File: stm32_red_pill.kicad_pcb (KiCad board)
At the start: 4 copper layers, 59 x 31 mm, 30 parts, among them J1 USB_B_Micro, J2 Conn_01x18, J3 Conn_01x18, J4 Conn_02x02_Top_Bottom, U1 STM32F103C8T6, U2 AMS1117-3.3, Y1 16MHZ

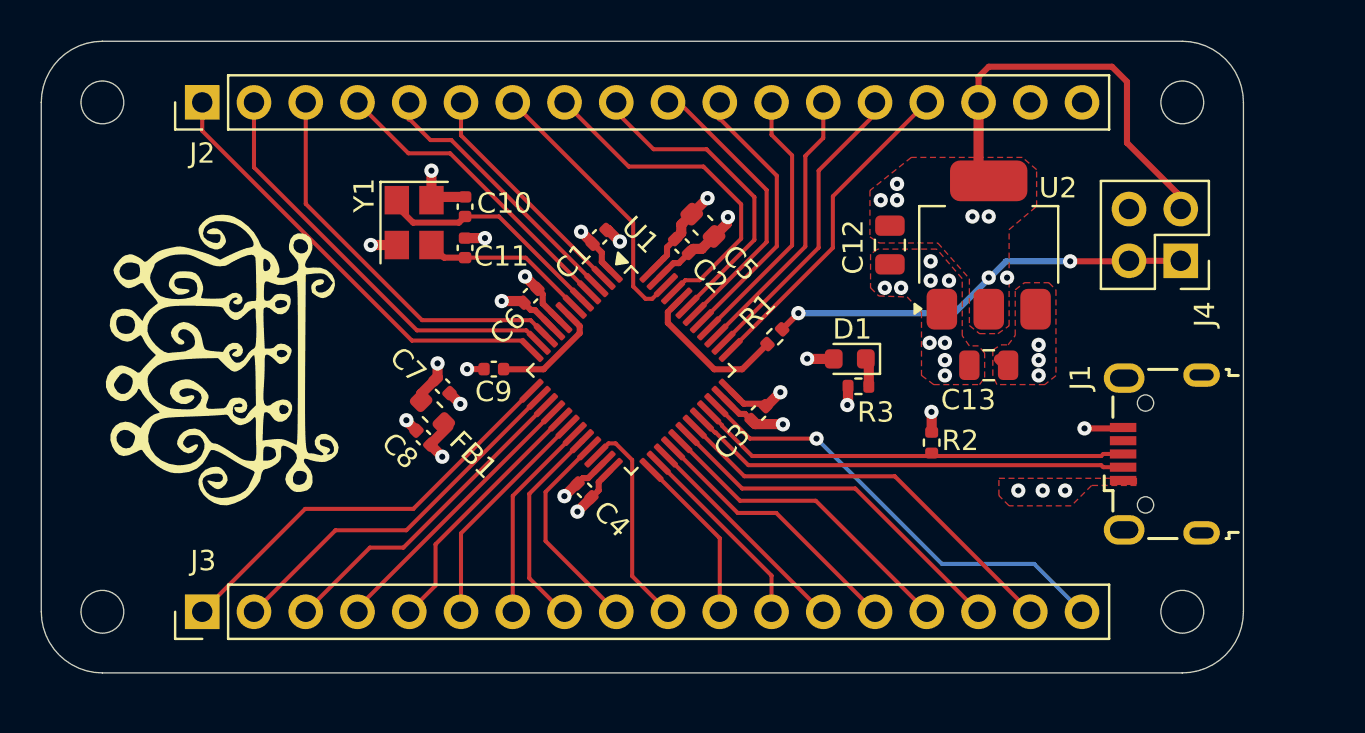
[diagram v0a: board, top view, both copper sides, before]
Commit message: lol
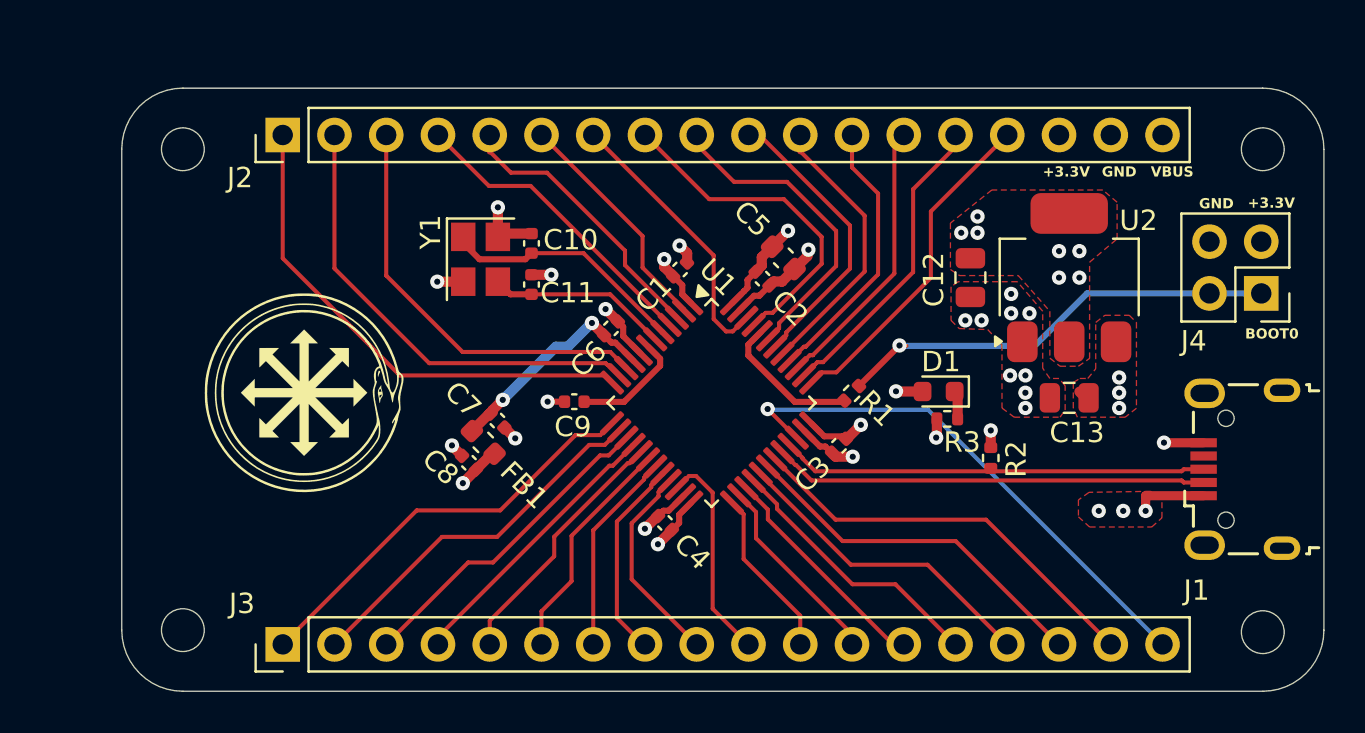
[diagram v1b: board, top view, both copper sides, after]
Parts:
- removed the G*** at (89.0, 101.7)
- added G*** (x2): LOGO, LOGO, F.Cu at (92.9, 103.2)
- D1: value BLUE -> RED
- moved R1 4.68 mm to (119.8, 103.3)
- moved D1 4.64 mm to (124.0, 103.2)
- moved R3 4.64 mm to (124.5, 104.5)
- moved H1 4.57 mm to (87.0, 91.3)
- moved H2 4.57 mm to (139.9, 91.3)
- moved C2 4.26 mm to (115.4, 97.7)
- moved C9 4.26 mm to (106.2, 103.7)
- moved C3 4.26 mm to (119.2, 105.8)
- moved C4 4.26 mm to (110.6, 109.6)
- moved C5 4.26 mm to (116.4, 96.6)
- moved C6 4.26 mm to (108.0, 100.1)
- moved U1 4.26 mm to (112.9, 103.8)
- moved C1 4.26 mm to (111.3, 97.2)
- moved C12 4.26 mm to (125.6, 97.6)
- moved C13 4.26 mm to (130.4, 103.5)
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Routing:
- net +3.3V: track 38.0 -> 18.4 mm
- net /PA13: track 22.6 -> 26.6 mm
- net VBUS: track 13.4 -> 17.0 mm
- net /PA2: track 22.0 -> 24.7 mm
- net /PA1: track 20.7 -> 22.7 mm
- net +3.3VA: track 9.66 -> 11.0 mm
- net /PA0: track 20.2 -> 21.3 mm
- net /SW_BOOT0: track 21.3 -> 22.2 mm, vias 2 -> 1
- net /BOOT0: track 7.74 -> 7.08 mm
- net /HSE_OUT: track 8.29 -> 8.90 mm
- net /HSE_IN: track 11.5 -> 12.1 mm
- net GND: track 25.4 -> 24.8 mm
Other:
- board size 59 x 31 mm -> 59 x 29.6 mm
- board text added: "+3.3V"
- board text added: "BOOT0"
- board text added: "GND"
- board text added: "STM32 Chaos Pill V1.0 Designed by Philip Perpetual Chaos"
- board text added: "VBUS"
- board text removed: "Designed by Philip V1.0"
